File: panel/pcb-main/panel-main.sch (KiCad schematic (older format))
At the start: 24 parts, among them J1 PSU IN, J2 SPEED CTRL, J3 ICSP, J4 PUSH-BUTTON, J5 DISPLAY, J6 CONN-L1, J7 CONN-L2, J8 CONN-R1, J9 CONN-R2, U1 LM7805, U8 PIC16F877A, Y1 20MHz

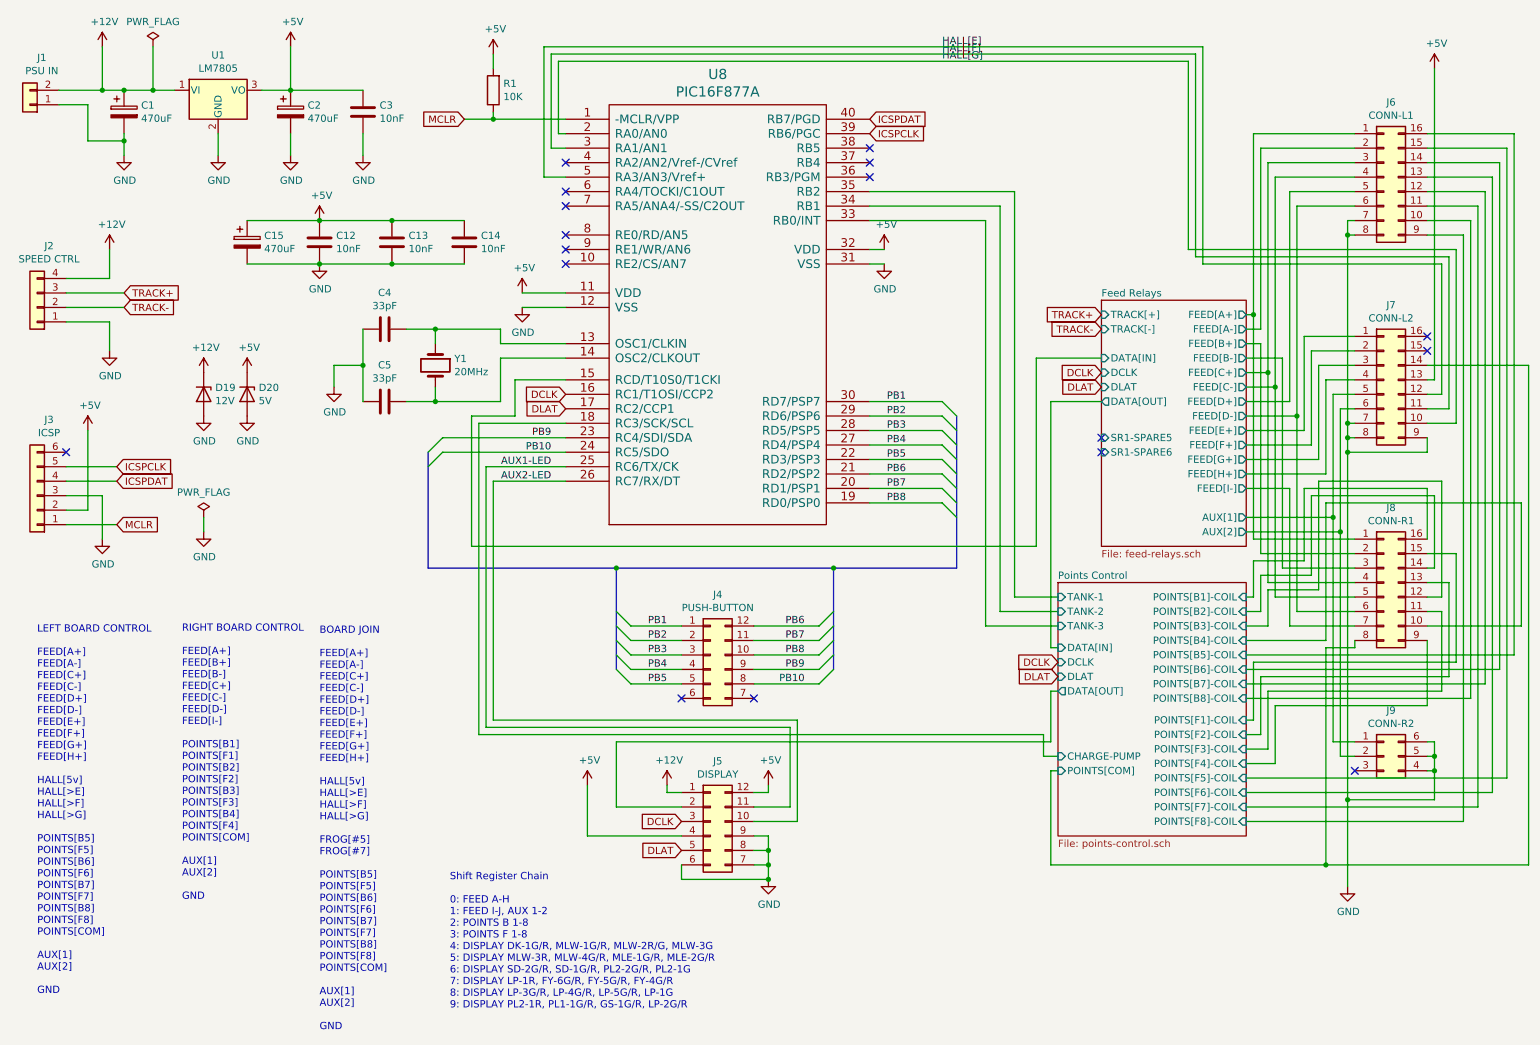
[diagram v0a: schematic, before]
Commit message: Completed all PCBs and added gerber files
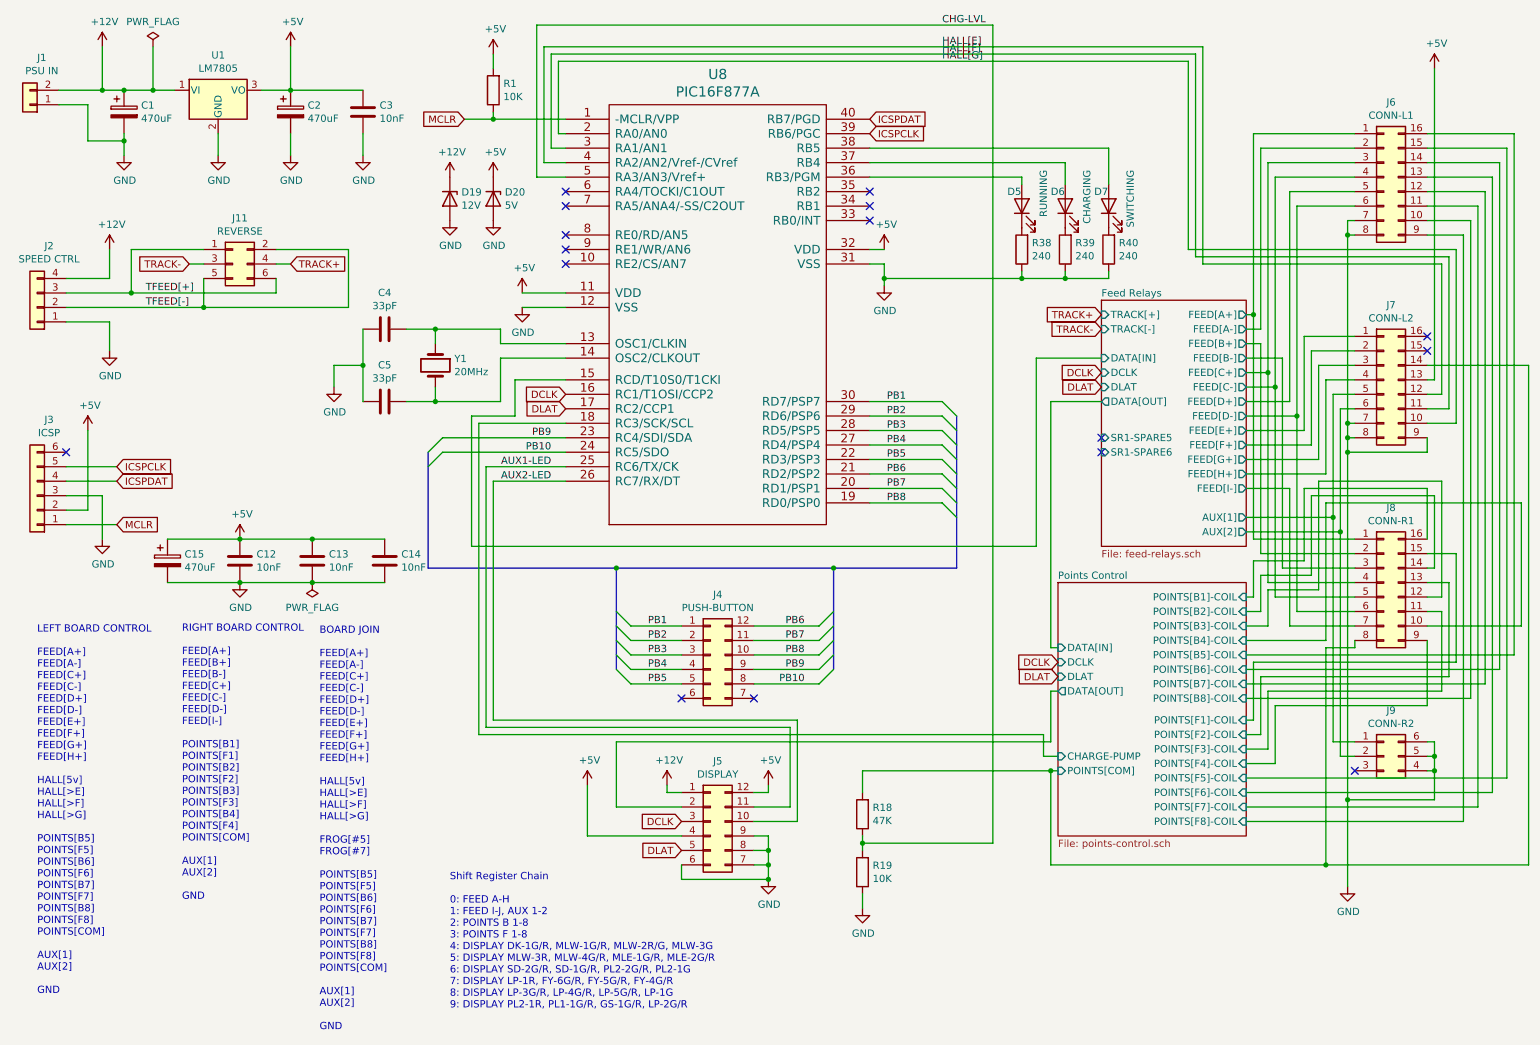
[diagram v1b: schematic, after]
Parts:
- added D5: RUNNING, LEDs:LED_D5.0mm, symbol Device:LED
- added D6: CHARGING, LEDs:LED_D5.0mm, symbol Device:LED
- added D7: SWITCHING, LEDs:LED_D5.0mm, symbol Device:LED
- added J11: REVERSE, Pin_Headers:Pin_Header_Straight_2x03_Pitch2.54mm, symbol Connector_Generic:Conn_02x03_Odd_Even
- added R18: 47K, Resistors_THT:R_Axial_DIN0207_L6.3mm_D2.5mm_P10.16mm_Horizontal, symbol Device:R
- added R19: 10K, Resistors_THT:R_Axial_DIN0207_L6.3mm_D2.5mm_P10.16mm_Horizontal, symbol Device:R
- added R38, R39, R40: 240, Resistors_THT:R_Axial_DIN0207_L6.3mm_D2.5mm_P10.16mm_Horizontal, symbol Device:R
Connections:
- net GND: now also R19.1, R38.1, R39.1, R40.1
- net HALL[E]: now also U8.4 (RA2/AN2/Vref-/CVref); no longer U8.5 (RA3/AN3/Vref+)
- net Points Control/POINTS[COM]: now also R18.2
- net TRACK+: now also J11.4 (Pin_4); no longer J2.3 (Pin_3)
- net TRACK-: now also J11.3 (Pin_3); no longer J2.2 (Pin_2)
- net at U8.36 (RB3/PGM): now also D5.2 (A)
- net at U8.37 (RB4): now also D6.2 (A)
- net at U8.38 (RB5): now also D7.2 (A)
- net Points Control/TANK-1: no longer names the net of U8.35 (RB2)
- net Points Control/TANK-2: no longer names the net of U8.34 (RB1)
- net Points Control/TANK-3: no longer names the net of U8.33 (RB0/INT)
- new net: D7.1 (K), R40.2
- new net: D6.1 (K), R39.2
- new net: D5.1 (K), R38.2
- new net CHG-LVL: R18.1, R19.2, U8.5 (RA3/AN3/Vref+)
- new net TFEED[+]: J11.1 (Pin_1), J11.6 (Pin_6), J2.3 (Pin_3)
- new net TFEED[-]: J11.2 (Pin_2), J11.5 (Pin_5), J2.2 (Pin_2)
- no-connect marks 17 -> 16
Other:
- moved on the sheet: C12, C13, C14, C15, D19, D20
